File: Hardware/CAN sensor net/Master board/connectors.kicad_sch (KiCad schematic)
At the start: 18 parts, among them J1 Micro_SD_Card_Con, J2 USB_B_Micro, J3 Conn_02x05_SWD, J5 532610671, J6 532610671, J7 530470310, U2 USBLC6-2SC6

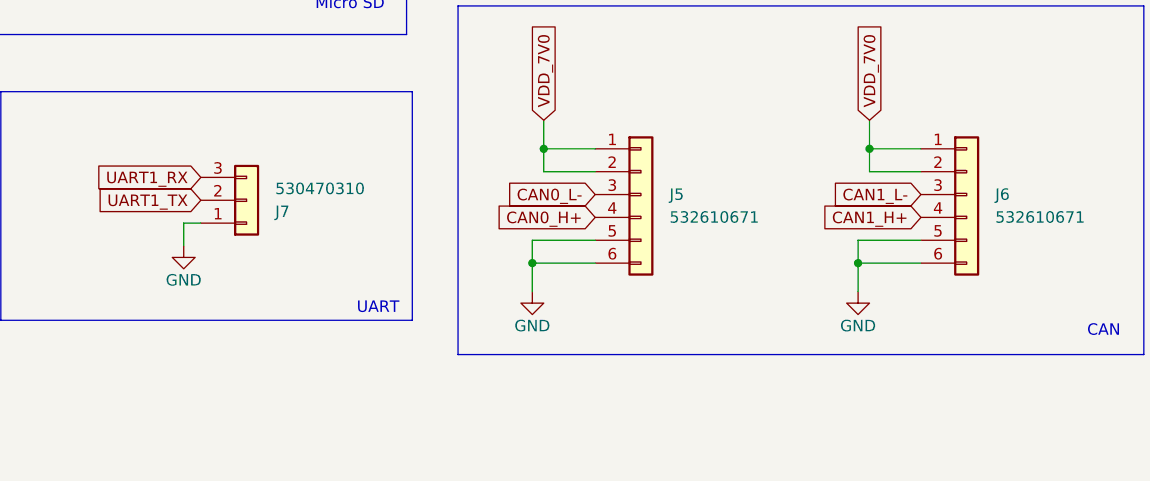
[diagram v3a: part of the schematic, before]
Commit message: Piezo fixes
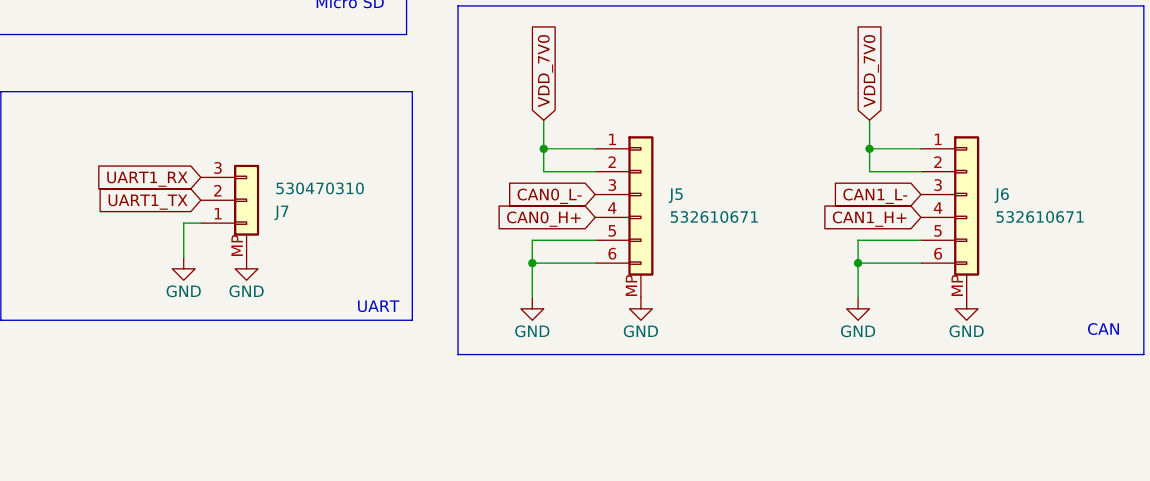
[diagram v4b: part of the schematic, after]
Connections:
- net GND: now also J5.MP, J6.MP, J7.MP
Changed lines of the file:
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@@
 	(wire
 		(pts
-			(xy 121.285 103.505) (xy 121.285 106.045)
+			(xy 121.285 103.505) (xy 121.285 107.315)
 		)
 		(stroke
@@
 	(wire
 		(pts
-			(xy 160.02 111.125) (xy 160.02 107.95)
+			(xy 160.02 111.76) (xy 160.02 107.95)
 		)
 		(stroke
@@
 	(wire
 		(pts
-			(xy 196.215 111.125) (xy 196.215 107.95)
+			(xy 196.215 111.76) (xy 196.215 107.95)
 		)
 		(stroke
@@
 	)
 	(symbol
+		(lib_name "Conn_01x06_1")
 		(lib_id "Connector_Generic:Conn_01x06")
 		(at 172.085 100.33 0)
@@
 		(pin "1"
 		)
+		(pin "MP"
+		)
 		(instances
 			(project "Master board"
@@
 	(symbol
 		(lib_id "power:GND")
-		(at 160.02 111.125 0)
+		(at 208.28 111.76 0)
+		(unit 1)
+		(exclude_from_sim no)
+		(in_bom yes)
+		(on_board yes)
+		(dnp no)
+		(property "Reference" "#PWR020"
+			(at 208.28 118.11 0)
+			(effects
+				(font
+					(size 1.27 1.27)
+				)
+				(hide yes)
+			)
+		)
+		(property "Value" "GND"
+			(at 208.28 115.57 0)
+			(effects
+				(font
+					(size 1.27 1.27)
+				)
+			)
+		)
+		(property "Footprint" ""
+			(at 208.28 111.76 0)
+			(effects
+				(font
+					(size 1.27 1.27)
+				)
+				(hide yes)
+			)
+		)
+		(property "Datasheet" ""
+			(at 208.28 111.76 0)
+			(effects
+				(font
+					(size 1.27 1.27)
+				)
+				(hide yes)
+			)
+		)
+		(property "Description" ""
+			(at 208.28 111.76 0)
+			(effects
+				(font
+					(size 1.27 1.27)
+				)
+				(hide yes)
+			)
+		)
+		(pin "1"
+		)
+		(instances
+			(project "Master board"
+				(path "/11ca9491-ebda-4c18-be98-3e552caaabb4/b817a2d8-bdd2-4de0-9d33-c531bafe0dc5"
+					(reference "#PWR020")
+					(unit 1)
+				)
+			)
+		)
+	)
+	(symbol
+		(lib_id "power:GND")
+		(at 160.02 111.76 0)
 		(unit 1)
 		(exclude_from_sim no)
@@
 		(dnp no)
 		(property "Reference" "#PWR014"
-			(at 160.02 117.475 0)
+			(at 160.02 118.11 0)
 			(effects
 				(font
@@
 		)
 		(property "Value" "GND"
-			(at 160.02 114.935 0)
+			(at 160.02 115.57 0)
 			(effects
 				(font
@@
 		)
 		(property "Footprint" ""
-			(at 160.02 111.125 0)
+			(at 160.02 111.76 0)
 			(effects
 				(font
@@
 		)
 		(property "Datasheet" ""
-			(at 160.02 111.125 0)
+			(at 160.02 111.76 0)
 			(effects
 				(font
@@
 		)
 		(property "Description" ""
-			(at 160.02 111.125 0)
+			(at 160.02 111.76 0)
 			(effects
 				(font
@@
 	)
 	(symbol
+		(lib_id "power:GND")
+		(at 172.085 111.76 0)
+		(unit 1)
+		(exclude_from_sim no)
+		(in_bom yes)
+		(on_board yes)
+		(dnp no)
+		(property "Reference" "#PWR010"
+			(at 172.085 118.11 0)
+			(effects
+				(font
+					(size 1.27 1.27)
+				)
+				(hide yes)
+			)
+		)
+		(property "Value" "GND"
+			(at 172.085 115.57 0)
+			(effects
+				(font
+					(size 1.27 1.27)
+				)
+			)
+		)
+		(property "Footprint" ""
+			(at 172.085 111.76 0)
+			(effects
+				(font
+					(size 1.27 1.27)
+				)
+				(hide yes)
+			)
+		)
+		(property "Datasheet" ""
+			(at 172.085 111.76 0)
+			(effects
+				(font
+					(size 1.27 1.27)
+				)
+				(hide yes)
+			)
+		)
+		(property "Description" ""
+			(at 172.085 111.76 0)
+			(effects
+				(font
+					(size 1.27 1.27)
+				)
+				(hide yes)
+			)
+		)
+		(pin "1"
+		)
+		(instances
+			(project "Master board"
+				(path "/11ca9491-ebda-4c18-be98-3e552caaabb4/b817a2d8-bdd2-4de0-9d33-c531bafe0dc5"
+					(reference "#PWR010")
+					(unit 1)
+				)
+			)
+		)
+	)
+	(symbol
 		(lib_id "Connector:USB_B_Micro")
 		(at 172.085 52.07 0)
@@
 		(lib_name "GND_1")
 		(lib_id "power:GND")
-		(at 121.285 106.045 0)
+		(at 121.285 107.315 0)
 		(unit 1)
 		(exclude_from_sim no)
@@
 		(dnp no)
 		(property "Reference" "#PWR09"
-			(at 121.285 112.395 0)
+			(at 121.285 113.665 0)
 			(effects
 				(font
@@
 		)
 		(property "Value" "GND"
-			(at 121.285 109.855 0)
+			(at 121.285 111.125 0)
 			(effects
 				(font
@@
 		)
 		(property "Footprint" ""
-			(at 121.285 106.045 0)
+			(at 121.285 107.315 0)
 			(effects
 				(font
@@
 		)
 		(property "Datasheet" ""
-			(at 121.285 106.045 0)
+			(at 121.285 107.315 0)
 			(effects
 				(font
@@
 		)
 		(property "Description" "Power symbol creates a global label with name \"GND\" , ground"
-			(at 121.285 106.045 0)
+			(at 121.285 107.315 0)
 			(effects
 				(font
@@
 	(symbol
 		(lib_id "power:GND")
-		(at 196.215 111.125 0)
+		(at 196.215 111.76 0)
 		(unit 1)
 		(exclude_from_sim no)
@@
 		(dnp no)
 		(property "Reference" "#PWR015"
-			(at 196.215 117.475 0)
+			(at 196.215 118.11 0)
 			(effects
 				(font
@@
 		)
 		(property "Value" "GND"
-			(at 196.215 114.935 0)
+			(at 196.215 115.57 0)
 			(effects
 				(font
@@
 		)
 		(property "Footprint" ""
-			(at 196.215 111.125 0)
+			(at 196.215 111.76 0)
 			(effects
 				(font
@@
 		)
 		(property "Datasheet" ""
-			(at 196.215 111.125 0)
+			(at 196.215 111.76 0)
 			(effects
 				(font
@@
 		)
 		(property "Description" ""
-			(at 196.215 111.125 0)
+			(at 196.215 111.76 0)
 			(effects
 				(font
@@
 		(pin "1"
 		)
+		(pin "MP"
+		)
 		(instances
 			(project "Master board"
@@
 	)
 	(symbol
+		(lib_name "GND_1")
+		(lib_id "power:GND")
+		(at 128.27 107.315 0)
+		(unit 1)
+		(exclude_from_sim no)
+		(in_bom yes)
+		(on_board yes)
+		(dnp no)
+		(property "Reference" "#PWR021"
+			(at 128.27 113.665 0)
+			(effects
+				(font
+					(size 1.27 1.27)
+				)
+				(hide yes)
+			)
+		)
+		(property "Value" "GND"
+			(at 128.27 111.125 0)
+			(effects
+				(font
+					(size 1.27 1.27)
+				)
+			)
+		)
+		(property "Footprint" ""
+			(at 128.27 107.315 0)
+			(effects
+				(font
+					(size 1.27 1.27)
+				)
+				(hide yes)
+			)
+		)
+		(property "Datasheet" ""
+			(at 128.27 107.315 0)
+			(effects
+				(font
+					(size 1.27 1.27)
+				)
+				(hide yes)
+			)
+		)
+		(property "Description" "Power symbol creates a global label with name \"GND\" , ground"
+			(at 128.27 107.315 0)
+			(effects
+				(font
+					(size 1.27 1.27)
+				)
+				(hide yes)
+			)
+		)
+		(pin "1"
+		)
+		(instances
+			(project "Master board"
+				(path "/11ca9491-ebda-4c18-be98-3e552caaabb4/b817a2d8-bdd2-4de0-9d33-c531bafe0dc5"
+					(reference "#PWR021")
+					(unit 1)
+				)
+			)
+		)
+	)
+	(symbol
 		(lib_id "Connector_Generic:Conn_01x03")
 		(at 128.27 100.965 0)
@@
 		(pin "1"
 		)
+		(pin "MP"
+		)
 		(instances

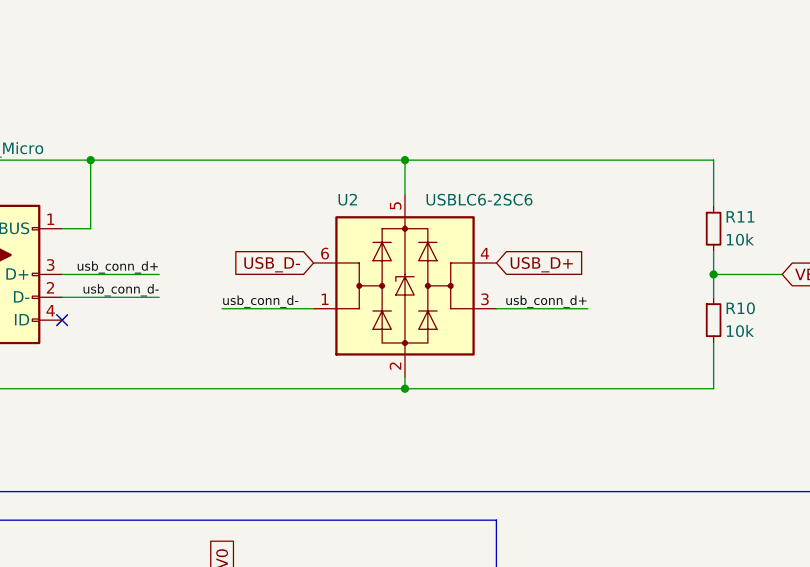
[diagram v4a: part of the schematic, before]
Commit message: Master board pre-production
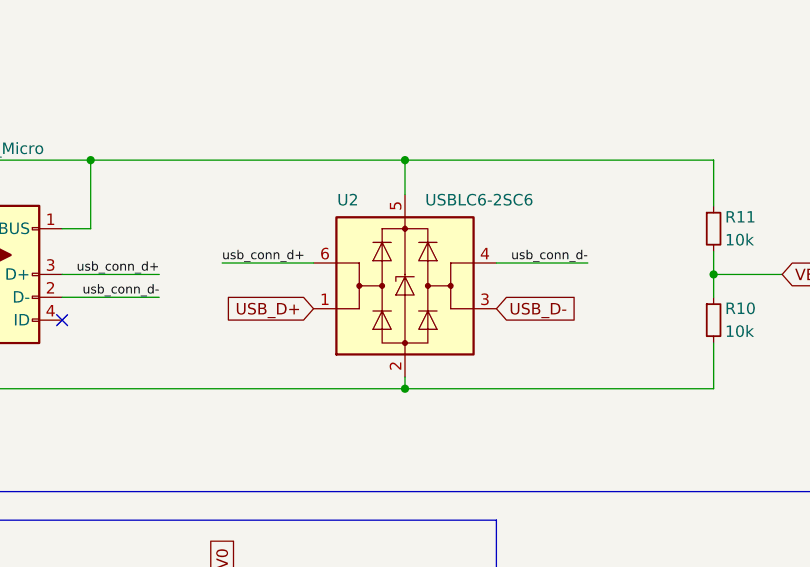
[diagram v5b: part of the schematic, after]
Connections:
- net USB_D+: now also U2.1 (I/O1); no longer U2.4 (I/O2)
- net USB_D-: now also U2.3 (I/O2); no longer U2.6 (I/O1)
- net usb_conn_d+: now also U2.6 (I/O1); no longer U2.3 (I/O2)
- net usb_conn_d-: now also U2.4 (I/O2); no longer U2.1 (I/O1)
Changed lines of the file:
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@@
-	(wire
-		(pts
-			(xy 238.125 55.88) (xy 227.965 55.88)
-		)
-		(stroke
-			(width 0)
-			(type default)
-		)
-	)
 	(wire
 		(pts
@@
 	(wire
 		(pts
+			(xy 197.485 50.8) (xy 207.645 50.8)
+		)
+		(stroke
+			(width 0)
+			(type default)
+		)
+	)
+	(wire
+		(pts
 			(xy 91.44 48.895) (xy 85.09 48.895)
 		)
@@
 		)
 	)
+	(wire
+		(pts
+			(xy 238.125 50.8) (xy 227.965 50.8)
+		)
+		(stroke
+			(width 0)
+			(type default)
+		)
+	)
 	(polyline
 		(pts
@@
 		(pts
 			(xy 34.29 43.815) (xy 69.215 43.815)
-		)
-		(stroke
-			(width 0)
-			(type default)
-		)
-	)
-	(wire
-		(pts
-			(xy 197.485 55.88) (xy 207.645 55.88)
 		)
 		(stroke
@@
 	)
 	(label "usb_conn_d+"
-		(at 238.125 55.88 180)
+		(at 197.485 50.8 0)
 		(fields_autoplaced yes)
 		(effects
@@
 				(size 1 1)
 			)
+			(justify left bottom)
+		)
+	)
+	(label "usb_conn_d-"
+		(at 238.125 50.8 180)
+		(fields_autoplaced yes)
+		(effects
+			(font
+				(size 1 1)
+			)
 			(justify right bottom)
-		)
-	)
-	(label "usb_conn_d-"
-		(at 197.485 55.88 0)
-		(fields_autoplaced yes)
-		(effects
-			(font
-				(size 1 1)
-			)
-			(justify left bottom)
 		)
 	)
@@
 	(global_label "USB_D+"
 		(shape input)
-		(at 227.965 50.8 0)
+		(at 207.645 55.88 180)
+		(fields_autoplaced yes)
+		(effects
+			(font
+				(size 1.27 1.27)
+			)
+			(justify right)
+		)
+		(property "Intersheetrefs" "${INTERSHEET_REFS}"
+			(at 197.0398 55.88 0)
+			(effects
+				(font
+					(size 1.27 1.27)
+				)
+				(justify right)
+				(hide yes)
+			)
+		)
+	)
+	(global_label "SDIO_D2"
+		(shape input)
+		(at 34.29 41.275 180)
+		(fields_autoplaced yes)
+		(effects
+			(font
+				(size 1.27 1.27)
+			)
+			(justify right)
+		)
+		(property "Intersheetrefs" "${INTERSHEET_REFS}"
+			(at 23.4429 41.275 0)
+			(effects
+				(font
+					(size 1.27 1.27)
+				)
+				(justify right)
+				(hide yes)
+			)
+		)
+	)
+	(global_label "UART1_TX"
+		(shape input)
+		(at 123.19 100.965 180)
+		(fields_autoplaced yes)
+		(effects
+			(font
+				(size 1.27 1.27)
+			)
+			(justify right)
+		)
+		(property "Intersheetrefs" "${INTERSHEET_REFS}"
+			(at 111.1939 100.965 0)
+			(effects
+				(font
+					(size 1.27 1.27)
+				)
+				(justify right)
+				(hide yes)
+			)
+		)
+	)
+	(global_label "DEBUG_SWDIO"
+		(shape input)
+		(at 57.785 108.585 0)
 		(fields_autoplaced yes)
 		(effects
@@
 		)
 		(property "Intersheetrefs" "${INTERSHEET_REFS}"
-			(at 238.5702 50.8 0)
+			(at 73.8935 108.585 0)
 			(effects
 				(font
@@
 		)
 	)
-	(global_label "SDIO_D2"
-		(shape input)
-		(at 34.29 41.275 180)
+	(global_label "NRST"
+		(shape input)
+		(at 57.785 118.745 0)
+		(fields_autoplaced yes)
+		(effects
+			(font
+				(size 1.27 1.27)
+			)
+			(justify left)
+		)
+		(property "Intersheetrefs" "${INTERSHEET_REFS}"
+			(at 65.5478 118.745 0)
+			(effects
+				(font
+					(size 1.27 1.27)
+				)
+				(justify left)
+				(hide yes)
+			)
+		)
+	)
+	(global_label "DEBUG_SWCLK"
+		(shape input)
+		(at 57.785 111.125 0)
+		(fields_autoplaced yes)
+		(effects
+			(font
+				(size 1.27 1.27)
+			)
+			(justify left)
+		)
+		(property "Intersheetrefs" "${INTERSHEET_REFS}"
+			(at 74.2563 111.125 0)
+			(effects
+				(font
+					(size 1.27 1.27)
+				)
+				(justify left)
+				(hide yes)
+			)
+		)
+	)
+	(global_label "CAN1_L-"
+		(shape input)
+		(at 203.2 100.33 180)
 		(fields_autoplaced yes)
 		(effects
@@
 		)
 		(property "Intersheetrefs" "${INTERSHEET_REFS}"
-			(at 23.4429 41.275 0)
+			(at 191.7481 100.33 0)
 			(effects
 				(font
@@
 		)
 	)
-	(global_label "UART1_TX"
-		(shape input)
-		(at 123.19 100.965 180)
-		(fields_autoplaced yes)
-		(effects
-			(font
-				(size 1.27 1.27)
-			)
-			(justify right)
-		)
-		(property "Intersheetrefs" "${INTERSHEET_REFS}"
-			(at 111.1939 100.965 0)
-			(effects
-				(font
-					(size 1.27 1.27)
-				)
-				(justify right)
-				(hide yes)
-			)
-		)
-	)
-	(global_label "DEBUG_SWDIO"
-		(shape input)
-		(at 57.785 108.585 0)
+	(global_label "USB_D-"
+		(shape input)
+		(at 227.965 55.88 0)
 		(fields_autoplaced yes)
 		(effects
@@
 		)
 		(property "Intersheetrefs" "${INTERSHEET_REFS}"
-			(at 73.8935 108.585 0)
+			(at 238.5702 55.88 0)
 			(effects
 				(font
@@
 				(hide yes)
 			)
-		)
-	)
-	(global_label "NRST"
-		(shape input)
-		(at 57.785 118.745 0)
-		(fields_autoplaced yes)
-		(effects
-			(font
-				(size 1.27 1.27)
-			)
-			(justify left)
-		)
-		(property "Intersheetrefs" "${INTERSHEET_REFS}"
-			(at 65.5478 118.745 0)
-			(effects
-				(font
-					(size 1.27 1.27)
-				)
-				(justify left)
-				(hide yes)
-			)
-		)
-	)
-	(global_label "DEBUG_SWCLK"
-		(shape input)
-		(at 57.785 111.125 0)
-		(fields_autoplaced yes)
-		(effects
-			(font
-				(size 1.27 1.27)
-			)
-			(justify left)
-		)
-		(property "Intersheetrefs" "${INTERSHEET_REFS}"
-			(at 74.2563 111.125 0)
-			(effects
-				(font
-					(size 1.27 1.27)
-				)
-				(justify left)
-				(hide yes)
-			)
-		)
-	)
-	(global_label "CAN1_L-"
-		(shape input)
-		(at 203.2 100.33 180)
-		(fields_autoplaced yes)
-		(effects
-			(font
-				(size 1.27 1.27)
-			)
-			(justify right)
-		)
-		(property "Intersheetrefs" "${INTERSHEET_REFS}"
-			(at 191.7481 100.33 0)
-			(effects
-				(font
-					(size 1.27 1.27)
-				)
-				(justify right)
-				(hide yes)
-			)
-		)
-	)
-	(global_label "USB_D-"
-		(shape input)
-		(at 207.645 50.8 180)
-		(fields_autoplaced yes)
-		(effects
-			(font
-				(size 1.27 1.27)
-			)
-			(justify right)
-		)
-		(property "Intersheetrefs" "${INTERSHEET_REFS}"
-			(at 197.0398 50.8 0)
-			(effects
-				(font
-					(size 1.27 1.27)
-				)
-				(justify right)
-				(hide yes)
-			)
